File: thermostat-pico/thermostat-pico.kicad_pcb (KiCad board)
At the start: 2 copper layers, 40 x 30 mm, 22 parts, among them J1 VAC IN, J2 CTRL, J3 UART, U1 LY68L6400SLIT, U2 ESP32-PICO-D4, U3 LM358DR2G, U4 TPS5430DDA, U5 TPS5430DDA

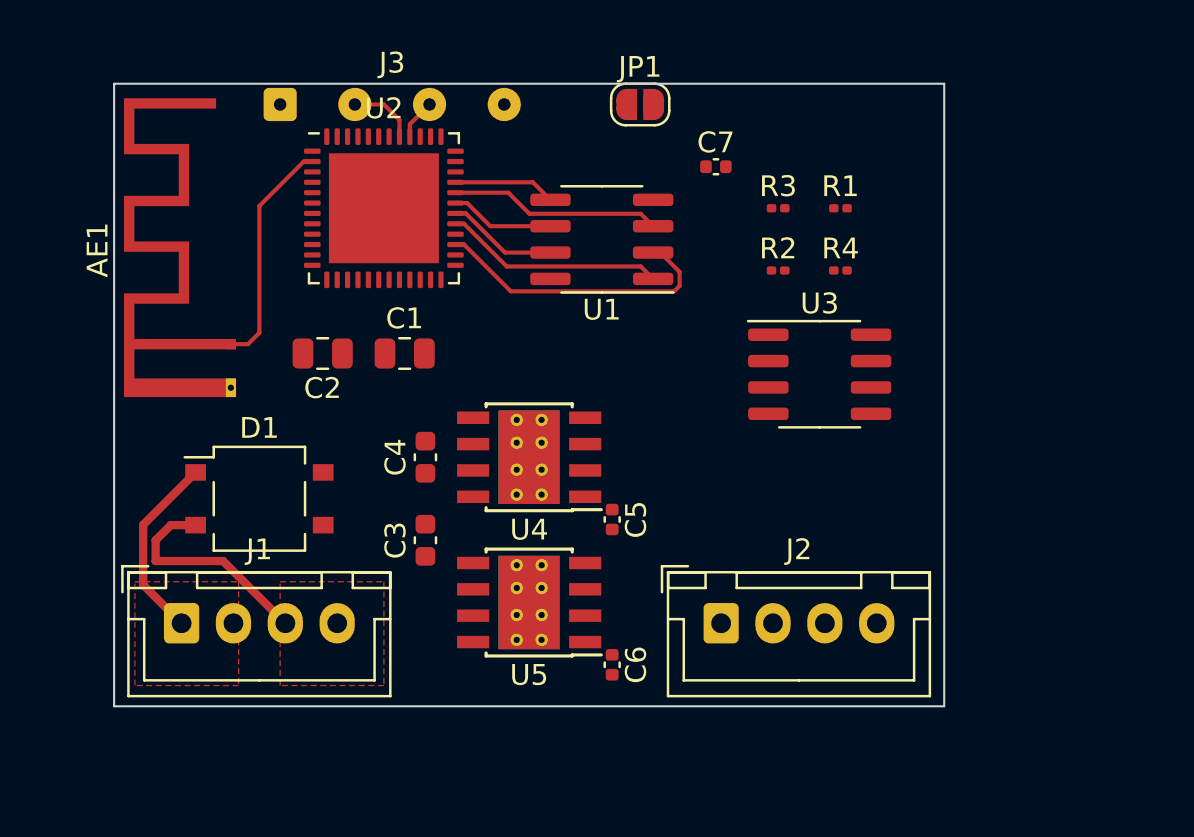
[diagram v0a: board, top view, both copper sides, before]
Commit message: Should be finished
Maybe the antenna could be different
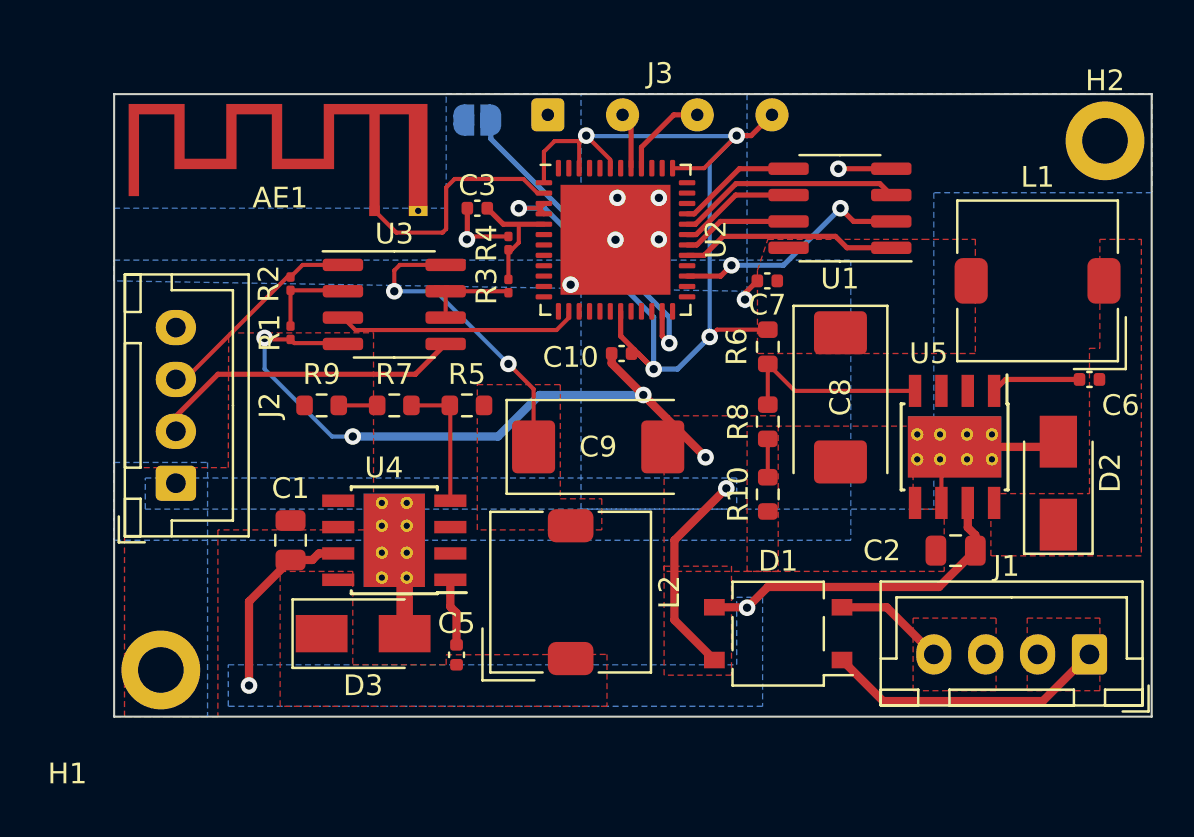
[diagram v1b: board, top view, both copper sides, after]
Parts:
- removed C4: 0.1uF/50V, Capacitor_SMD:C_0603_1608Metric
- added C10: 0.01uF, Capacitor_SMD:C_0402_1005Metric, F.Cu at (107.5, 99.0)
- added C8: 470uF/6.3V, Capacitor_Tantalum_SMD:CP_EIA-7343-31_Kemet-D, F.Cu at (118.0, 101.1)
- added C9: 470uF/6.3V, Capacitor_Tantalum_SMD:CP_EIA-7343-31_Kemet-D, F.Cu at (106.3, 103.5)
- added D2: SS34, Diode_SMD:D_SMA, F.Cu at (128.5, 105.2)
- added D3: SS34, Diode_SMD:D_SMA, F.Cu at (95.0, 112.5)
- added H1: MountingHole_Pad, MountingHole:MountingHole_2.2mm_M2_DIN965_Pad, F.Cu at (85.2, 114.2)
- added H2: MountingHole_Pad, MountingHole:MountingHole_2.2mm_M2_DIN965_Pad, F.Cu at (130.8, 88.8)
- added L1: 22uH, inductors:L_SXN_SMRH74-220MT, F.Cu at (127.5, 95.5)
- added L2: 22uH, inductors:L_SXN_SMRH74-220MT, F.Cu at (105.0, 110.5)
- added R10: 270, Resistor_SMD:R_0603_1608Metric, F.Cu at (114.5, 105.8)
- added R5: 10k, Resistor_SMD:R_0603_1608Metric, F.Cu at (100.0, 101.5)
- added R6: 10k, Resistor_SMD:R_0603_1608Metric, F.Cu at (114.5, 98.7)
- added R7: 1.1k, Resistor_SMD:R_0603_1608Metric, F.Cu at (96.5, 101.5)
- added R8: 5.6k, Resistor_SMD:R_0603_1608Metric, F.Cu at (114.5, 102.3)
- added R9: 33, Resistor_SMD:R_0603_1608Metric, F.Cu at (93.0, 101.5)
- AE1: value Antenna -> Antenna_Shield; footprint RF_Antenna:Texas_SWRA117D_2.4GHz_Right -> RF_Antenna:Texas_SWRA117D_2.4GHz_Left
- C3: value 0.1uF/50V -> 0.1uF; footprint Capacitor_SMD:C_0603_1608Metric -> Capacitor_SMD:C_0402_1005Metric
- C7: value 0.01uF -> 0.1uF
- JP1: moved to B.Cu
- moved J1 43.8 mm to (130.0, 113.5), turned to 180 degrees
- moved C2 31.9 mm to (123.5, 108.5)
- moved R1 27.2 mm to (91.5, 98.0), turned to -90 degrees
- moved J2 27.1 mm to (86.0, 105.2), turned to 90 degrees
- moved C6 26.8 mm to (130.0, 100.2), turned to 0 degrees
- moved D1 25.8 mm to (115.0, 112.5), turned to 180 degrees
- moved R2 23.5 mm to (91.5, 95.6), turned to 90 degrees
- moved U5 21.8 mm to (123.5, 103.5), turned to -90 degrees
- moved U3 20.8 mm to (96.5, 96.6)
- moved C3 16.2 mm to (100.5, 92.0), turned to 0 degrees
- moved R4 16.1 mm to (102.0, 93.7), turned to 90 degrees
- moved R3 13.5 mm to (102.0, 95.8), turned to 90 degrees
- moved J3 12.9 mm to (103.9, 87.5)
- moved U1 11.6 mm to (118.0, 92.0)
- moved U2 11.3 mm to (107.2, 93.5)
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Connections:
- net Net-(C5-Pad2) renamed /PH12
- net Net-(C6-Pad2) renamed /PH33
- AE1 pad 2: (no net) -> GND
- C1 pad 1: /REC_OUT -> /D1_OUT
- C2 pad 1: /REC_OUT -> /D1_OUT
- C3 pad 1: /REC_OUT -> GND
- C3 pad 2: GND -> /ADC1
- D1 pad 3: /REC_OUT -> /D1_OUT
- JP1 pad 1: unconnected-(JP1-Pad1) -> /BOOT
- JP1 pad 2: unconnected-(JP1-Pad2) -> GND
- R3 pad 2: Net-(R3-Pad2) -> /ADC1
- R4 pad 1: Net-(R3-Pad2) -> /ADC1
- U2 pad 1: Net-(U2-Pad1) -> /VCC33
- U2 pad 14: unconnected-(U2-Pad14) -> /DAC1
- U2 pad 15: unconnected-(U2-Pad15) -> /DAC2
- U2 pad 19: unconnected-(U2-Pad19) -> /VCC33
- U2 pad 23: unconnected-(U2-Pad23) -> /BOOT
- U2 pad 3: Net-(U2-Pad3) -> /VCC33
- U2 pad 37: unconnected-(U2-Pad37) -> /VCC33
- U2 pad 4: Net-(U2-Pad3) -> /VCC33
- U2 pad 43: Net-(U2-Pad1) -> /VCC33
- U2 pad 46: Net-(U2-Pad1) -> /VCC33
- U2 pad 5: unconnected-(U2-Pad5) -> /ADC1
- U2 pad 6: unconnected-(U2-Pad6) -> /ADC2
- U3 pad 3: unconnected-(U3-Pad3) -> /DAC1
- U3 pad 4: unconnected-(U3-Pad4) -> GND
- U3 pad 8: unconnected-(U3-Pad8) -> /VCC12
- U4 pad 4: unconnected-(U4-Pad4) -> Net-(R5-Pad2)
- U4 pad 7: /REC_OUT -> /D1_OUT
- U5 pad 4: unconnected-(U5-Pad4) -> Net-(R6-Pad2)
- U5 pad 7: /REC_OUT -> /D1_OUT
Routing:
- net GND: track 0.00 -> 60.1 mm, vias 0 -> 13
- net /VCC33: track 0.00 -> 55.2 mm, vias 0 -> 5
- net /D1_OUT: track 0.00 -> 25.5 mm, vias 0 -> 2
- net /BOOT: track 0.00 -> 16.0 mm, vias 0 -> 1
- net /VCC12: track 0.00 -> 15.0 mm, vias 0 -> 2
- net /CTRL0_IN: track 0.00 -> 14.4 mm
- net /DAC1: track 0.00 -> 11.7 mm
- net /CTRL0_OUT: track 0.00 -> 9.90 mm
- net Net-(R6-Pad2): track 0.00 -> 9.60 mm
- net Net-(R5-Pad2): track 0.00 -> 6.42 mm
- net /ADC1: track 0.00 -> 5.89 mm
- net /24VAC+: track 10.7 -> 5.37 mm
- net /24VAC-: track 9.08 -> 13.7 mm
- net Net-(C6-Pad1): track 0.00 -> 4.34 mm
- net Net-(R3-Pad1): track 0.00 -> 4.23 mm
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- added copper zone on B.Cu, net /D1_OUT
- added copper zone on F.Cu, net /PH12
- added copper zone on F.Cu, net /PH33
- added copper zone on F.Cu, net /VCC12
- added copper zone on F.Cu, net /VCC33
- added copper zone on B.Cu, net GND
- added copper zone on F.Cu, net GND
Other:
- board size 40 x 30 mm -> 50 x 30 mm
- board text added: "+"
- board text added: "-"
- board text added: "24VAC"
- board text added: "CTRL_IN"
- board text added: "CTRL_OUT"
- board text added: "GND"
- board text added: "URX"
- board text added: "UTX"
- board text added: "VCC"
